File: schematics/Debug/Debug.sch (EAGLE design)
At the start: 12 parts

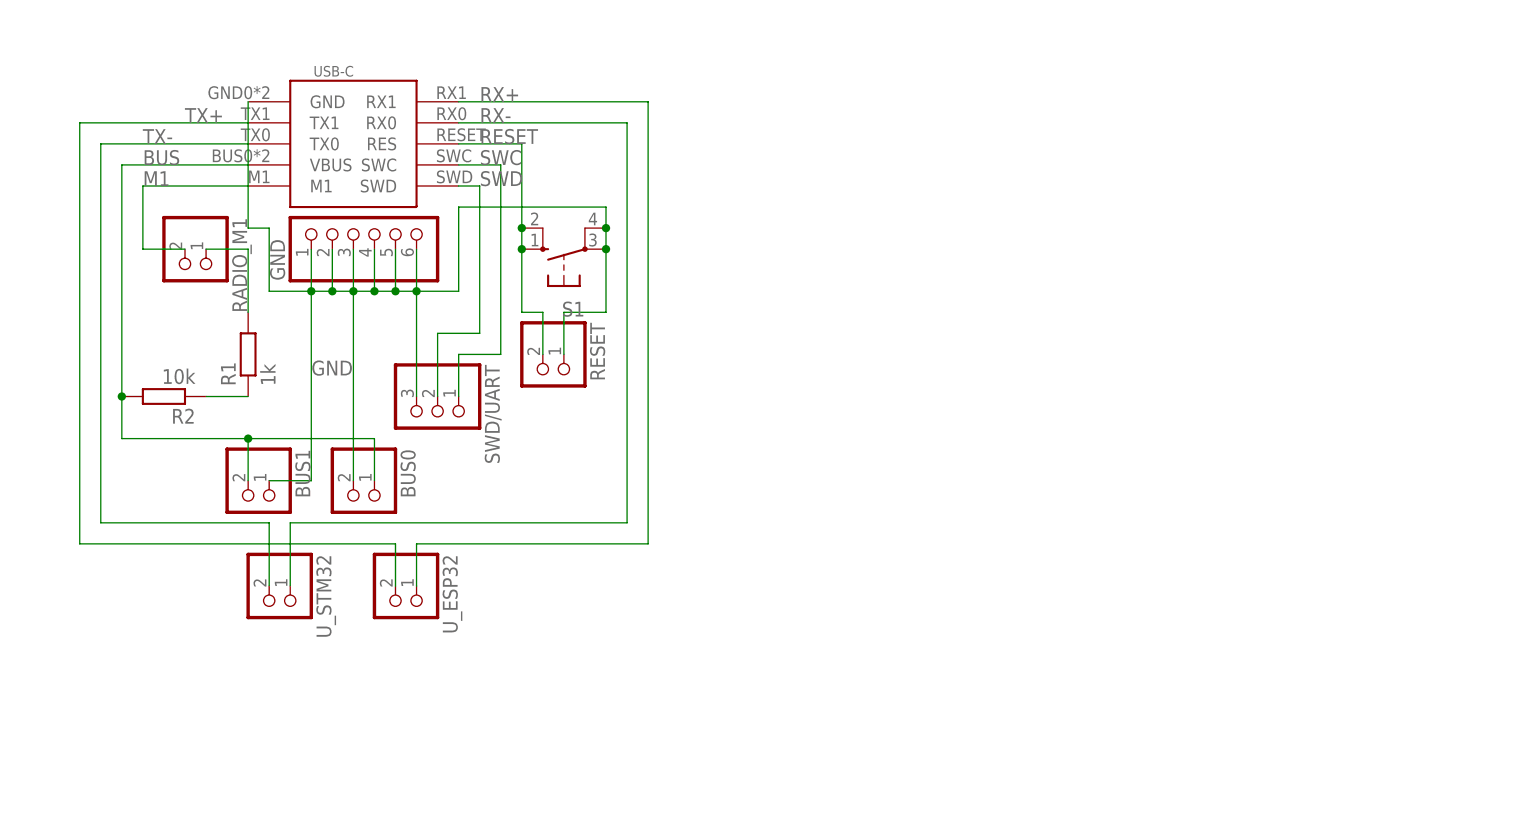
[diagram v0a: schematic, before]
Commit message: Очередная дебажная плата
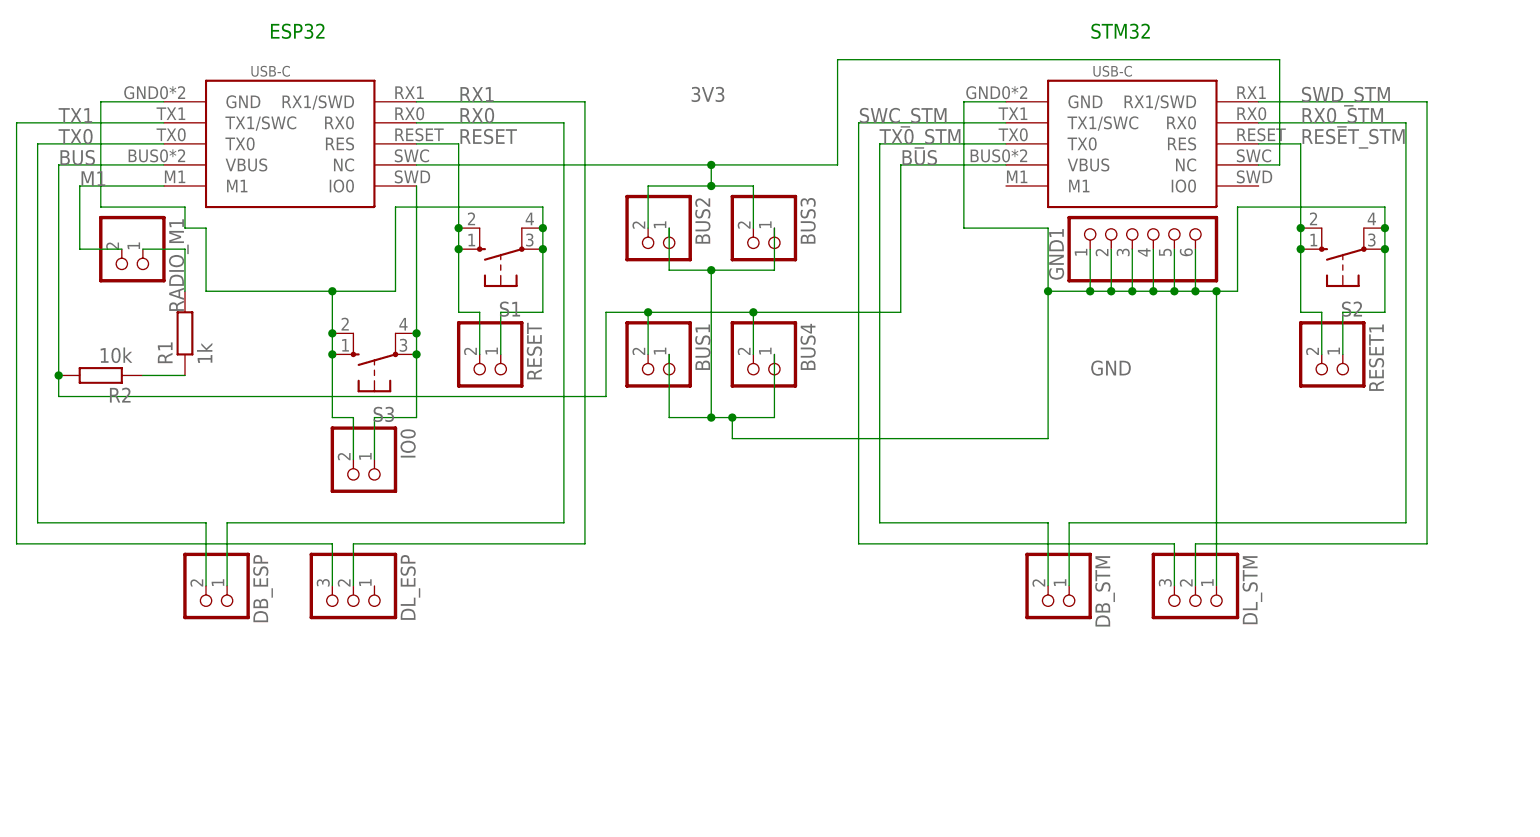
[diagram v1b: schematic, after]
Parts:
- removed BUS0, U_ESP32, U_STM32: (no value), pinhead:PINHD-1X2
- removed GND: (no value), pinhead:PINHD-1X6
- removed SWD/UART: (no value), pinhead:PINHD-1X3
- added BUS2, BUS3, BUS4, DB_ESP, DB_STM, IO0, RESET1: (no value), pinhead:PINHD-1X2
- added DL_ESP, DL_STM: (no value), pinhead:PINHD-1X3
- added GND1: (no value), pinhead:PINHD-1X6
- added S2, S3: (no value), switch-omron:10-XX
- added U$2: USB-C, CanCubeSat:USB-C
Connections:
- removed net RX+: U$1.RX1, U_ESP32.1
- removed net RX-: U$1.RX0, U_STM32.1
- removed net SWC: SWD/UART.1, U$1.SWC
- removed net SWD: SWD/UART.2, U$1.SWD
- removed net TX+: U$1.TX1, U_ESP32.2
- removed net TX-: U$1.TX0, U_STM32.2
- new net 3V3: BUS2.2, BUS3.2, U$1.NC, U$2.NC
- new net N$3: IO0.1, S3.P, S3.P1, U$1.IO0
- new net RESET_STM: RESET1.2, S2.S, S2.S1, U$2.RES
- new net RX0: DB_ESP.1, U$1.RX0
- new net RX0_STM: DB_STM.1, U$2.RX0
- new net RX1: DL_ESP.2, U$1.RX1/SWD
- new net SWC_STM: DL_STM.3, U$2.TX1/SWC
- new net SWD_STM: DL_STM.2, U$2.RX1/SWD
- new net TX0: DB_ESP.2, U$1.TX0
- new net TX0_STM: DB_STM.2, U$2.TX0
- new net TX1: DL_ESP.3, U$1.TX1/SWC
- net BUS: now also BUS4.2, U$2.VBUS; no longer BUS0.1
- net GND: now also BUS2.1, BUS3.1, BUS4.1, DL_STM.1, GND1.1, GND1.2, GND1.3, GND1.4, GND1.5, GND1.6, IO0.2, RESET1.1, S2.P, S2.P1, S3.S, S3.S1, U$2.GND; no longer BUS0.2, GND.1, GND.2, GND.3, GND.4, GND.5, GND.6, SWD/UART.3
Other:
- note added: "ESP32"
- note added: "STM32"
- moved on the sheet: BUS1, R1, R2, RADIO_M1, RESET, S1

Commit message: Отладочная плата v2
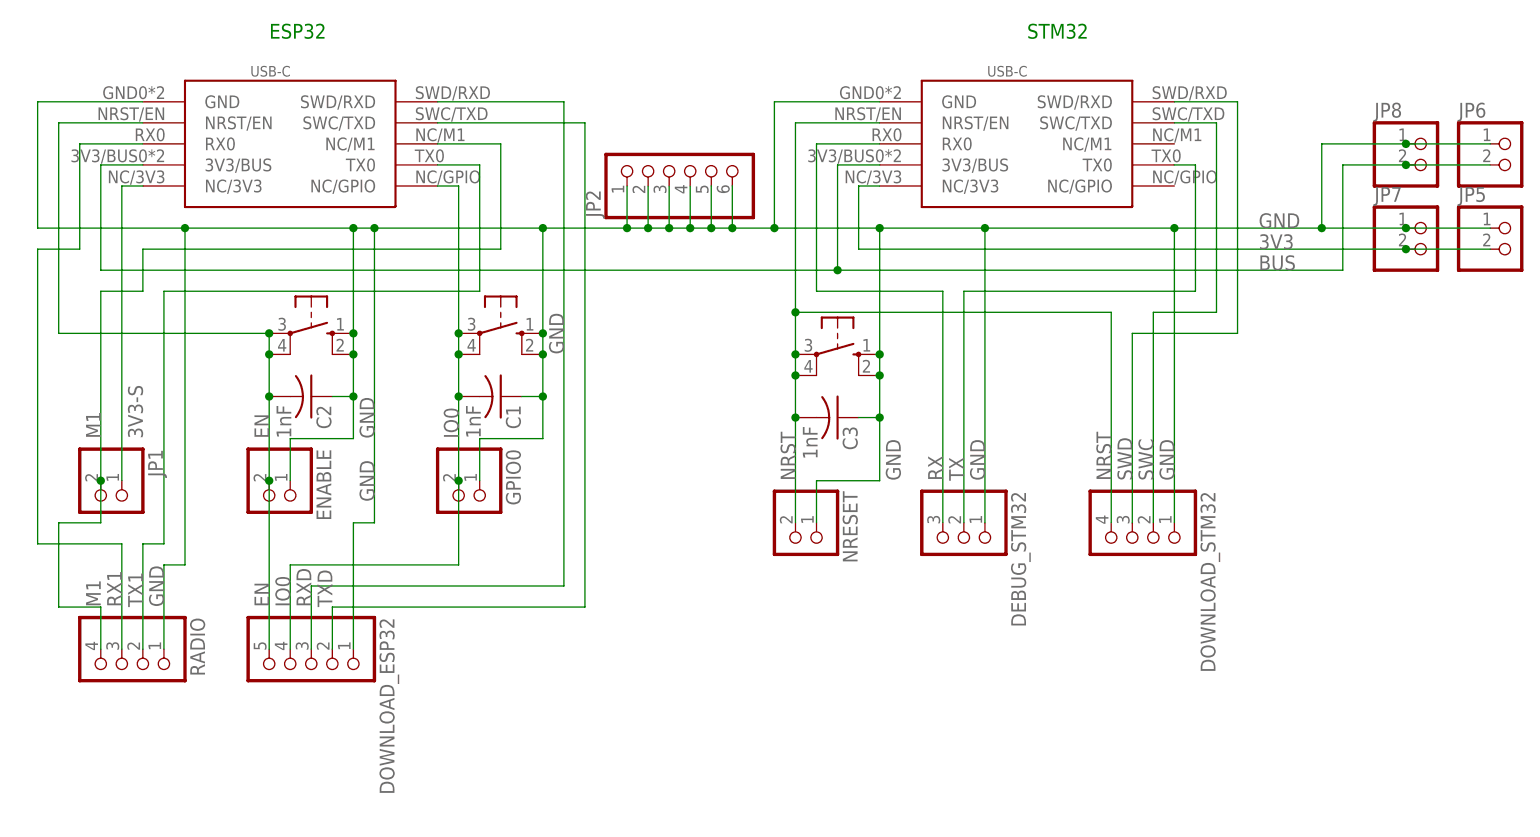
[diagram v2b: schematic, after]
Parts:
- removed BUS1, BUS2, BUS3, BUS4, DB_ESP, DB_STM, RADIO_M1, RESET, RESET1: (no value), pinhead:PINHD-1X2
- removed DL_ESP, DL_STM: (no value), pinhead:PINHD-1X3
- removed GND1: (no value), pinhead:PINHD-1X6
- removed R1: 1k, rcl:R-EU_R0603
- removed R2: 10k, rcl:R-EU_R0603
- removed S1, S2, S3: (no value), switch-omron:10-XX
- added C1, C2, C3: 1nF, rcl:C-USC0603
- added DEBUG_STM32: (no value), pinhead:PINHD-1X3
- added DOWNLOAD_ESP32: (no value), pinhead:PINHD-1X5
- added DOWNLOAD_STM32, RADIO: (no value), pinhead:PINHD-1X4
- added EN, NRST: (no value), switch-omron:10-XX
- added ENABLE, GPIO0, JP1, JP5, JP6, JP7, JP8, NRESET: (no value), pinhead:PINHD-1X2
- added JP2: (no value), pinhead:PINHD-1X6
- IO0: device pinhead:PINHD-1X2 -> switch-omron:10-XX
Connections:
- removed net N$3: IO0.1, S3.P, S3.P1, U$1.IO0
- removed net N$7: R1.2, RADIO_M1.1
- removed net N$8: R1.1, R2.1
- removed net RESET: RESET.2, S1.S, S1.S1, U$1.RES
- removed net RESET_STM: RESET1.2, S2.S, S2.S1, U$2.RES
- removed net RX0: DB_ESP.1, U$1.RX0
- removed net RX0_STM: DB_STM.1, U$2.RX0
- removed net SWC_STM: DL_STM.3, U$2.TX1/SWC
- removed net SWD_STM: DL_STM.2, U$2.RX1/SWD
- removed net TX0: DB_ESP.2, U$1.TX0
- removed net TX0_STM: DB_STM.2, U$2.TX0
- new net 3V3-S: JP1.1, U$1.NC/3V3
- new net EN: C2.2, DOWNLOAD_ESP32.5, EN.P, EN.P1, ENABLE.2, U$1.NRST/EN
- new net IO0: C1.2, DOWNLOAD_ESP32.4, GPIO0.2, IO0.P, IO0.P1, U$1.NC/GPIO
- new net NRST: C3.2, DOWNLOAD_STM32.4, NRESET.2, NRST.P, NRST.P1, U$2.NRST/EN
- new net RX: DEBUG_STM32.3, U$2.RX0
- new net RXD: DOWNLOAD_ESP32.3, U$1.SWD/RXD
- new net SWC: DOWNLOAD_STM32.2, U$2.SWC/TXD
- new net SWD: DOWNLOAD_STM32.3, U$2.SWD/RXD
- new net TX: DEBUG_STM32.2, U$2.TX0
- new net TXD: DOWNLOAD_ESP32.2, U$1.SWC/TXD
- net 3V3: now also JP5.2, JP7.2, U$2.NC/3V3; no longer BUS2.2, BUS3.2, U$1.NC, U$2.NC
- net BUS: now also JP6.2, JP8.2, U$1.3V3/BUS, U$2.3V3/BUS; no longer BUS1.2, BUS4.2, R2.2, U$1.VBUS, U$2.VBUS
- net GND: now also C1.1, C2.1, C3.1, DEBUG_STM32.1, DOWNLOAD_ESP32.1, DOWNLOAD_STM32.1, EN.S, EN.S1, ENABLE.1, GPIO0.1, IO0.S, IO0.S1, JP2.1, JP2.2, JP2.3, JP2.4, JP2.5, JP2.6, JP5.1, JP6.1, JP7.1, JP8.1, NRESET.1, NRST.S, NRST.S1, RADIO.1; no longer BUS1.1, BUS2.1, BUS3.1, BUS4.1, DL_STM.1, GND1.1, GND1.2, GND1.3, GND1.4, GND1.5, GND1.6, IO0.2, RESET.1, RESET1.1, S1.P, S1.P1, S2.P, S2.P1, S3.S, S3.S1
- net M1: now also JP1.2, RADIO.4, U$1.NC/M1; no longer RADIO_M1.2, U$1.M1
- net RX1: now also RADIO.3, U$1.RX0; no longer DL_ESP.2, U$1.RX1/SWD
- net TX1: now also RADIO.2, U$1.TX0; no longer DL_ESP.3, U$1.TX1/SWC
